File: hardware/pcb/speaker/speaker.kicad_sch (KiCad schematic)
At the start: 51 parts, among them J1 JST SH BM02B Connector, J2 JST SH BM02B Connector, J3 JST SH BM02B Connector, J4 JST SH BM02B Connector, J5 JST SH BM02B Connector, J6 JST SH BM02B Connector, J7 Conn_01x02, M1 Ultrasonic_Transducer, M10 Ultrasonic_Transducer, M11 Ultrasonic_Transducer, M12 Ultrasonic_Transducer, M13 Ultrasonic_Transducer, M14 Ultrasonic_Transducer, M15 Ultrasonic_Transducer, M16 Ultrasonic_Transducer, M17 Ultrasonic_Transducer, M18 Ultrasonic_Transducer, M19 Ultrasonic_Transducer, M2 Ultrasonic_Transducer, M3 Ultrasonic_Transducer, M4 Ultrasonic_Transducer, M5 Ultrasonic_Transducer, M6 Ultrasonic_Transducer, M7 Ultrasonic_Transducer, M8 Ultrasonic_Transducer, M9 Ultrasonic_Transducer, U1 LTC2631-Z, U2 LM2735XMF

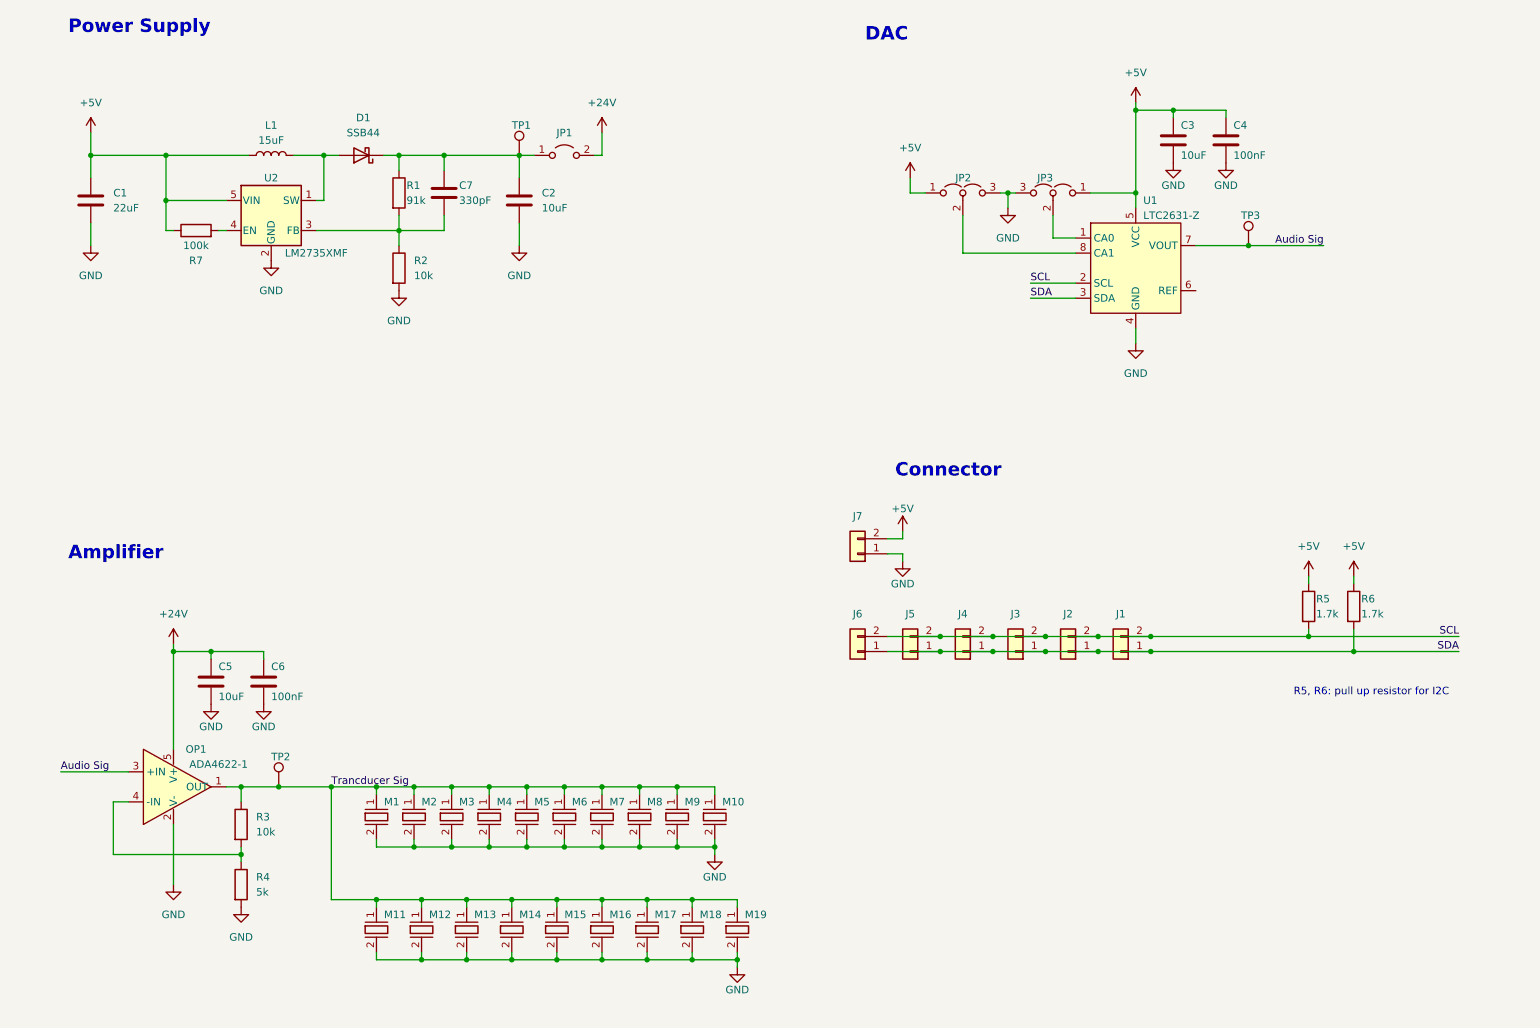
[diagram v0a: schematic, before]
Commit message: REWORK pcb design
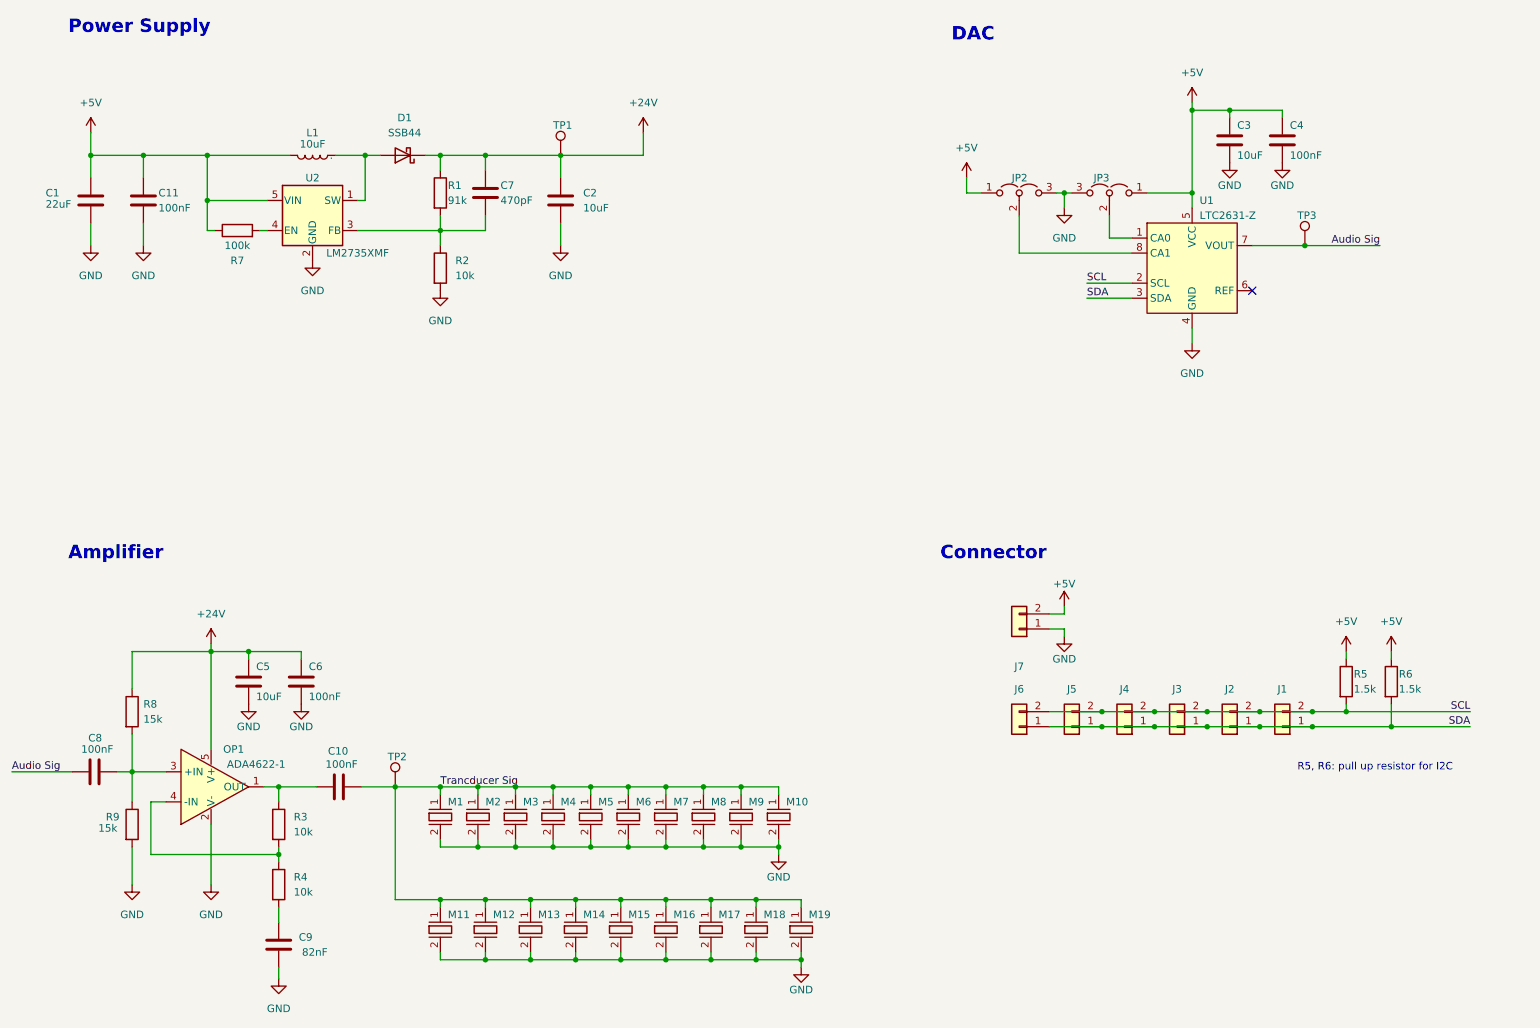
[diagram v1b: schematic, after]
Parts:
- removed JP1: Jumper_2_Open, Jumper:SolderJumper-2_P1.3mm_Bridged2Bar_Pad1.0x1.5mm, symbol Jumper:Jumper_2_Open
- added C10, C11, C8: 100nF, Capacitor_SMD:C_0805_2012Metric, symbol Device:C
- added C9: 82nF, Capacitor_SMD:C_0805_2012Metric, symbol Device:C
- added R8, R9: 15k, Resistor_SMD:R_0805_2012Metric, symbol Device:R
- C7: value 330pF -> 470pF
- L1: value 15uF -> 10uF; footprint Inductor_SMD:L_1206_3216Metric -> Inductor_SMD:L_Wuerth_5030_Handsolder; winding (none) -> .
- R4: value 5k -> 10k
- R5, R6: value 1.7k -> 1.5k
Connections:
- net +24V: now also C2.1, C7.1, D1.1 (K), R1.1, TP1.1, R8.1
- net +5V: now also L1.2, C11.1; no longer L1.1
- net Audio Sig: now also C8.1; no longer OP1.3 (+IN)
- net GND: now also C11.2, C9.1, R9.2; no longer R4.2
- net Trancducer Sig: now also C10.2; no longer OP1.1 (OUT), R3.1
- net at D1.2 (A), U2.1 (SW): now also L1.1; no longer L1.2
- new net: C8.2, OP1.3 (+IN), R8.2, R9.1
- new net: C9.2, R4.2
- new net: C10.1, OP1.1 (OUT), R3.1
- no-connect marks 0 -> 1
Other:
- moved on the sheet: C2, C3, C4, C5, C6, C7, D1, J1, J2, J3, J4, J5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
